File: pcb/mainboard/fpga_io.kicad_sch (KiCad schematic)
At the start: 3 parts, among them U1 XC6SLX-FTG256

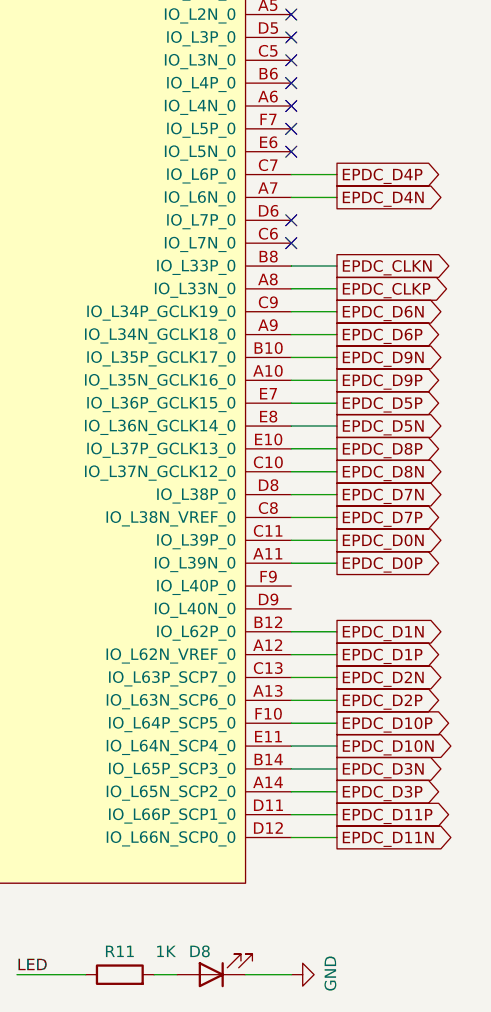
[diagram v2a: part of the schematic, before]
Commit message: PCB r0p11
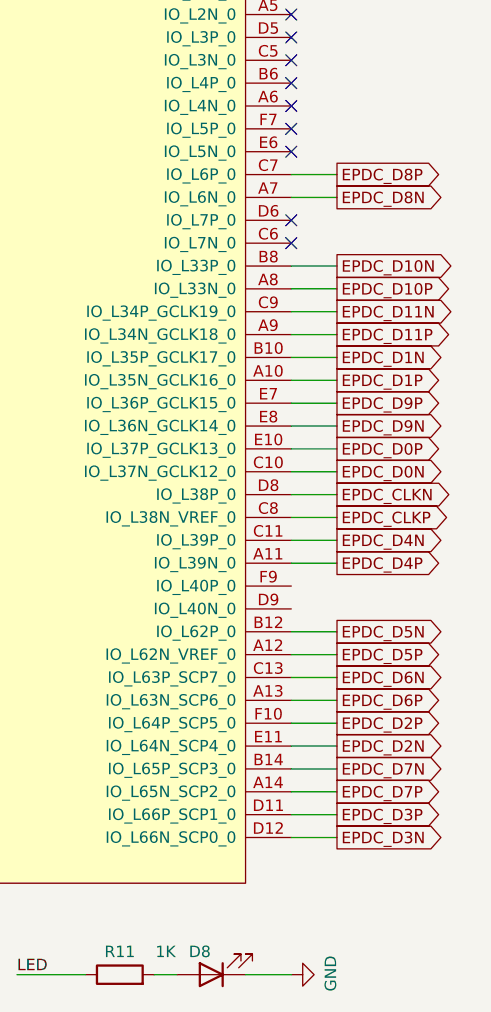
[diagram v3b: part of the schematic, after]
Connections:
- net EPDC_CLKN: now also U1.D8 (IO_L38P_0); no longer U1.B8 (IO_L33P_0)
- net EPDC_CLKP: now also U1.C8 (IO_L38N_VREF_0); no longer U1.A8 (IO_L33N_0)
- net EPDC_D0N: now also U1.C10 (IO_L37N_GCLK12_0); no longer U1.C11 (IO_L39P_0)
- net EPDC_D0P: now also U1.E10 (IO_L37P_GCLK13_0); no longer U1.A11 (IO_L39N_0)
- net EPDC_D10N: now also U1.B8 (IO_L33P_0); no longer U1.E11 (IO_L64N_SCP4_0)
- net EPDC_D10P: now also U1.A8 (IO_L33N_0); no longer U1.F10 (IO_L64P_SCP5_0)
- net EPDC_D11N: now also U1.C9 (IO_L34P_GCLK19_0); no longer U1.D12 (IO_L66N_SCP0_0)
- net EPDC_D11P: now also U1.A9 (IO_L34N_GCLK18_0); no longer U1.D11 (IO_L66P_SCP1_0)
- net EPDC_D1N: now also U1.B10 (IO_L35P_GCLK17_0); no longer U1.B12 (IO_L62P_0)
- net EPDC_D1P: now also U1.A10 (IO_L35N_GCLK16_0); no longer U1.A12 (IO_L62N_VREF_0)
- net EPDC_D2N: now also U1.E11 (IO_L64N_SCP4_0); no longer U1.C13 (IO_L63P_SCP7_0)
- net EPDC_D2P: now also U1.F10 (IO_L64P_SCP5_0); no longer U1.A13 (IO_L63N_SCP6_0)
- net EPDC_D3N: now also U1.D12 (IO_L66N_SCP0_0); no longer U1.B14 (IO_L65P_SCP3_0)
- net EPDC_D3P: now also U1.D11 (IO_L66P_SCP1_0); no longer U1.A14 (IO_L65N_SCP2_0)
- net EPDC_D4N: now also U1.C11 (IO_L39P_0); no longer U1.A7 (IO_L6N_0)
- net EPDC_D4P: now also U1.A11 (IO_L39N_0); no longer U1.C7 (IO_L6P_0)
- net EPDC_D5N: now also U1.B12 (IO_L62P_0); no longer U1.E8 (IO_L36N_GCLK14_0)
- net EPDC_D5P: now also U1.A12 (IO_L62N_VREF_0); no longer U1.E7 (IO_L36P_GCLK15_0)
- net EPDC_D6N: now also U1.C13 (IO_L63P_SCP7_0); no longer U1.C9 (IO_L34P_GCLK19_0)
- net EPDC_D6P: now also U1.A13 (IO_L63N_SCP6_0); no longer U1.A9 (IO_L34N_GCLK18_0)
- net EPDC_D7N: now also U1.B14 (IO_L65P_SCP3_0); no longer U1.D8 (IO_L38P_0)
- net EPDC_D7P: now also U1.A14 (IO_L65N_SCP2_0); no longer U1.C8 (IO_L38N_VREF_0)
- net EPDC_D8N: now also U1.A7 (IO_L6N_0); no longer U1.C10 (IO_L37N_GCLK12_0)
- net EPDC_D8P: now also U1.C7 (IO_L6P_0); no longer U1.E10 (IO_L37P_GCLK13_0)
- net EPDC_D9N: now also U1.E8 (IO_L36N_GCLK14_0); no longer U1.B10 (IO_L35P_GCLK17_0)
- net EPDC_D9P: now also U1.E7 (IO_L36P_GCLK15_0); no longer U1.A10 (IO_L35N_GCLK16_0)
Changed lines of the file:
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@@
 		)
 	)
-	(global_label "EPDC_D1N"
+	(global_label "EPDC_D5N"
 		(shape output)
 		(at 218.44 124.46 0)
@@
 		)
 	)
-	(global_label "EPDC_D1P"
+	(global_label "EPDC_D5P"
 		(shape output)
 		(at 218.44 127 0)
@@
 		)
 	)
-	(global_label "EPDC_D8P"
+	(global_label "EPDC_D0P"
 		(shape output)
 		(at 218.44 104.14 0)
@@
 		)
 	)
-	(global_label "EPDC_D3N"
+	(global_label "EPDC_D7N"
 		(shape output)
 		(at 218.44 139.7 0)
@@
 		)
 	)
-	(global_label "EPDC_D0P"
+	(global_label "EPDC_D4P"
 		(shape output)
 		(at 218.44 116.84 0)
@@
 		)
 	)
-	(global_label "EPDC_D3P"
+	(global_label "EPDC_D7P"
 		(shape output)
 		(at 218.44 142.24 0)
@@
 		)
 	)
-	(global_label "EPDC_D6P"
+	(global_label "EPDC_D11P"
 		(shape output)
 		(at 218.44 91.44 0)
@@
 		)
 		(property "Intersheetrefs" "${INTERSHEET_REFS}"
-			(at 231.1013 91.44 0)
+			(at 232.3108 91.44 0)
 			(effects
 				(font
@@
 		)
 	)
+	(global_label "EPDC_D2P"
+		(shape output)
+		(at 218.44 134.62 0)
+		(fields_autoplaced yes)
+		(effects
+			(font
+				(size 1.27 1.27)
+			)
+			(justify left)
+		)
+		(property "Intersheetrefs" "${INTERSHEET_REFS}"
+			(at 231.1013 134.62 0)
+			(effects
+				(font
+					(size 1.27 1.27)
+				)
+				(justify left)
+				(hide yes)
+			)
+		)
+	)
+	(global_label "DPI_VS"
+		(shape input)
+		(at 119.38 170.18 0)
+		(fields_autoplaced yes)
+		(effects
+			(font
+				(size 1.27 1.27)
+			)
+			(justify left)
+		)
+		(property "Intersheetrefs" "${INTERSHEET_REFS}"
+			(at 128.6963 170.18 0)
+			(effects
+				(font
+					(size 1.27 1.27)
+				)
+				(justify left)
+				(hide yes)
+			)
+		)
+	)
+	(global_label "FMC_NE1"
+		(shape input)
+		(at 119.38 149.86 0)
+		(fields_autoplaced yes)
+		(effects
+			(font
+				(size 1.27 1.27)
+			)
+			(justify left)
+		)
+		(property "Intersheetrefs" "${INTERSHEET_REFS}"
+			(at 130.8318 149.86 0)
+			(effects
+				(font
+					(size 1.27 1.27)
+				)
+				(justify left)
+				(hide yes)
+			)
+		)
+	)
 	(global_label "EPDC_D10P"
 		(shape output)
-		(at 218.44 134.62 0)
-		(fields_autoplaced yes)
-		(effects
-			(font
-				(size 1.27 1.27)
-			)
-			(justify left)
-		)
-		(property "Intersheetrefs" "${INTERSHEET_REFS}"
-			(at 232.3108 134.62 0)
-			(effects
-				(font
-					(size 1.27 1.27)
-				)
-				(justify left)
-				(hide yes)
-			)
-		)
-	)
-	(global_label "DPI_VS"
-		(shape input)
-		(at 119.38 170.18 0)
-		(fields_autoplaced yes)
-		(effects
-			(font
-				(size 1.27 1.27)
-			)
-			(justify left)
-		)
-		(property "Intersheetrefs" "${INTERSHEET_REFS}"
-			(at 128.6963 170.18 0)
-			(effects
-				(font
-					(size 1.27 1.27)
-				)
-				(justify left)
-				(hide yes)
-			)
-		)
-	)
-	(global_label "FMC_NE1"
-		(shape input)
-		(at 119.38 149.86 0)
-		(fields_autoplaced yes)
-		(effects
-			(font
-				(size 1.27 1.27)
-			)
-			(justify left)
-		)
-		(property "Intersheetrefs" "${INTERSHEET_REFS}"
-			(at 130.8318 149.86 0)
-			(effects
-				(font
-					(size 1.27 1.27)
-				)
-				(justify left)
-				(hide yes)
-			)
-		)
-	)
-	(global_label "EPDC_CLKP"
-		(shape output)
 		(at 218.44 86.36 0)
 		(fields_autoplaced yes)
@@
 		)
 		(property "Intersheetrefs" "${INTERSHEET_REFS}"
-			(at 232.1899 86.36 0)
+			(at 232.3108 86.36 0)
 			(effects
 				(font
@@
 		)
 	)
-	(global_label "EPDC_D11N"
+	(global_label "EPDC_D3N"
 		(shape output)
 		(at 218.44 147.32 0)
@@
 		)
 		(property "Intersheetrefs" "${INTERSHEET_REFS}"
-			(at 232.3713 147.32 0)
+			(at 231.1618 147.32 0)
 			(effects
 				(font
@@
 		)
 	)
-	(global_label "EPDC_D8N"
+	(global_label "EPDC_D0N"
 		(shape output)
 		(at 218.44 106.68 0)
@@
 		)
 	)
-	(global_label "EPDC_D5N"
+	(global_label "EPDC_D9N"
 		(shape output)
 		(at 218.44 101.6 0)
@@
 		)
 	)
-	(global_label "EPDC_D9N"
+	(global_label "EPDC_D1N"
 		(shape output)
 		(at 218.44 93.98 0)
@@
 		)
 	)
-	(global_label "EPDC_CLKN"
+	(global_label "EPDC_D10N"
 		(shape output)
 		(at 218.44 83.82 0)
@@
 		)
 		(property "Intersheetrefs" "${INTERSHEET_REFS}"
-			(at 232.2504 83.82 0)
+			(at 232.3713 83.82 0)
 			(effects
 				(font
@@
 		)
 	)
-	(global_label "EPDC_D5P"
+	(global_label "EPDC_D9P"
 		(shape output)
 		(at 218.44 99.06 0)
@@
 		)
 	)
-	(global_label "EPDC_D2N"
+	(global_label "EPDC_D6N"
 		(shape output)
 		(at 218.44 129.54 0)
@@
 		)
 	)
-	(global_label "EPDC_D0N"
+	(global_label "EPDC_D4N"
 		(shape output)
 		(at 218.44 114.3 0)
@@
 		)
 	)
-	(global_label "EPDC_D2P"
+	(global_label "EPDC_D6P"
 		(shape output)
 		(at 218.44 132.08 0)
@@
 		)
 	)
-	(global_label "EPDC_D4N"
+	(global_label "EPDC_D8N"
 		(shape output)
 		(at 218.44 76.2 0)
@@
 		)
 	)
-	(global_label "EPDC_D7N"
+	(global_label "EPDC_CLKN"
 		(shape output)
 		(at 218.44 109.22 0)
@@
 		)
 		(property "Intersheetrefs" "${INTERSHEET_REFS}"
-			(at 231.1618 109.22 0)
+			(at 232.2504 109.22 0)
 			(effects
 				(font
@@
 		)
 	)
-	(global_label "EPDC_D6N"
+	(global_label "EPDC_D11N"
 		(shape output)
 		(at 218.44 88.9 0)
@@
 		)
 		(property "Intersheetrefs" "${INTERSHEET_REFS}"
-			(at 231.1618 88.9 0)
+			(at 232.3713 88.9 0)
 			(effects
 				(font
@@
 		)
 	)
-	(global_label "EPDC_D9P"
+	(global_label "EPDC_D1P"
 		(shape output)
 		(at 218.44 96.52 0)
@@
 		)
 	)
-	(global_label "EPDC_D4P"
+	(global_label "EPDC_D8P"
 		(shape output)
 		(at 218.44 73.66 0)
@@
 		)
 	)
-	(global_label "EPDC_D7P"
+	(global_label "EPDC_CLKP"
 		(shape output)
 		(at 218.44 111.76 0)
@@
 		)
 		(property "Intersheetrefs" "${INTERSHEET_REFS}"
-			(at 231.1013 111.76 0)
-			(effects
-				(font
-					(size 1.27 1.27)
-				)
-				(justify left)
-				(hide yes)
-			)
-		)
-	)
-	(global_label "EPDC_D11P"
+			(at 232.1899 111.76 0)
+			(effects
+				(font
+					(size 1.27 1.27)
+				)
+				(justify left)
+				(hide yes)
+			)
+		)
+	)
+	(global_label "EPDC_D3P"
 		(shape output)
 		(at 218.44 144.78 0)
@@
 		)
 		(property "Intersheetrefs" "${INTERSHEET_REFS}"
-			(at 232.3108 144.78 0)
+			(at 231.1013 144.78 0)
 			(effects
 				(font
@@
 		)
 	)
-	(global_label "EPDC_D10N"
+	(global_label "EPDC_D2N"
 		(shape output)
 		(at 218.44 137.16 0)
@@
 		)
 		(property "Intersheetrefs" "${INTERSHEET_REFS}"
-			(at 232.3713 137.16 0)
-			(effects
-				(font
+			(at 231.1618 137.16 0)
+			(effects
+				(font

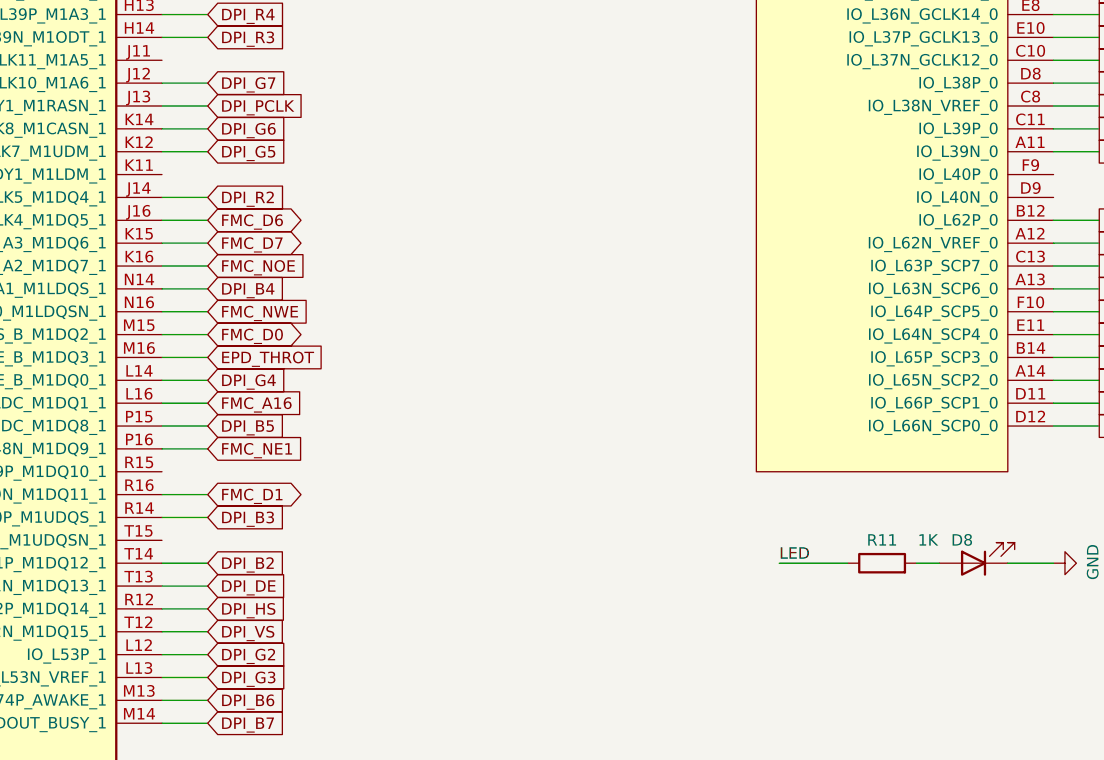
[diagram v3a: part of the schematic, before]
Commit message: PCB r0p13
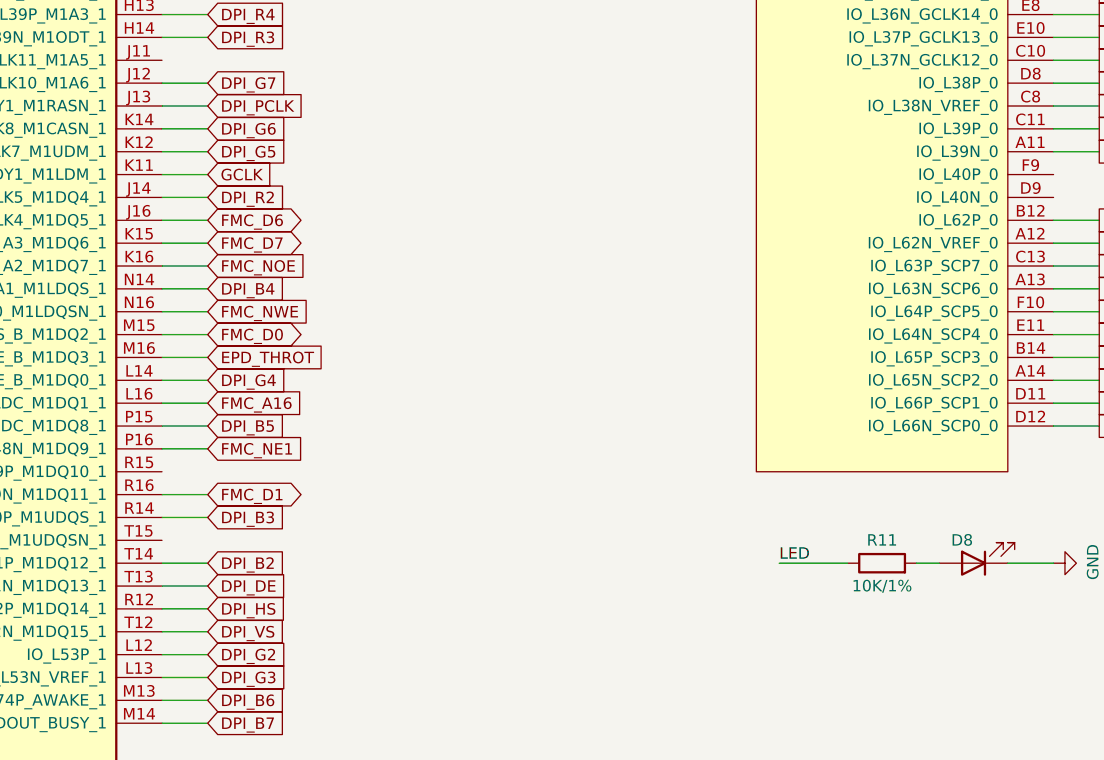
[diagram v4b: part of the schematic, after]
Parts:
- R11: value 1K -> 10K/1%
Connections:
- net GCLK: now reaches U1.K11 (IO_L42N_GCLK6_TRDY1_M1LDM_1)
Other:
- company: (none) -> Copyright 2025 Wenting Zhang
- title: (none) -> Glider
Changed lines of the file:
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@@
 	(generator_version "8.0")
 	(paper "A4")
+	(title_block
+		(title "Glider")
+		(date "2025-04-18")
+		(rev "R0.13")
+		(company "Copyright 2025 Wenting Zhang")
+	)
 	(junction
 		(at 101.6 25.4)
@@
 	(wire
 		(pts
+			(xy 119.38 119.38) (xy 114.3 119.38)
+		)
+		(stroke
+			(width 0)
+			(type default)
+		)
+	)
+	(wire
+		(pts
 			(xy 119.38 50.8) (xy 114.3 50.8)
 		)
@@
 		)
 	)
+	(global_label "GCLK"
+		(shape input)
+		(at 119.38 119.38 0)
+		(fields_autoplaced yes)
+		(effects
+			(font
+				(size 1.27 1.27)
+			)
+			(justify left)
+		)
+		(property "Intersheetrefs" "${INTERSHEET_REFS}"
+			(at 126.6312 119.3006 0)
+			(effects
+				(font
+					(size 1.27 1.27)
+				)
+				(justify left)
+				(hide yes)
+			)
+		)
+	)
 	(global_label "FMC_D0"
 		(shape bidirectional)
@@
 			)
 		)
-		(property "Value" "1K"
-			(at 199.39 160.02 90)
+		(property "Value" "10K/1%"
+			(at 194.31 165.1 90)
 			(effects
 				(font
